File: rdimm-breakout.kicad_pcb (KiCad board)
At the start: 10 copper layers, 152.9 x 45 mm, 33 parts, among them IC1 MIC5317-2.5YM5-TR, IC2 MIC5225-3.3YM5-TR, J1 WE_629105150521, J4 0022232041, U1 FT2232HL-REEL, U14 2199155-1, U8 PCA9517ADMR2G, Y1 KX-7_12,MHz

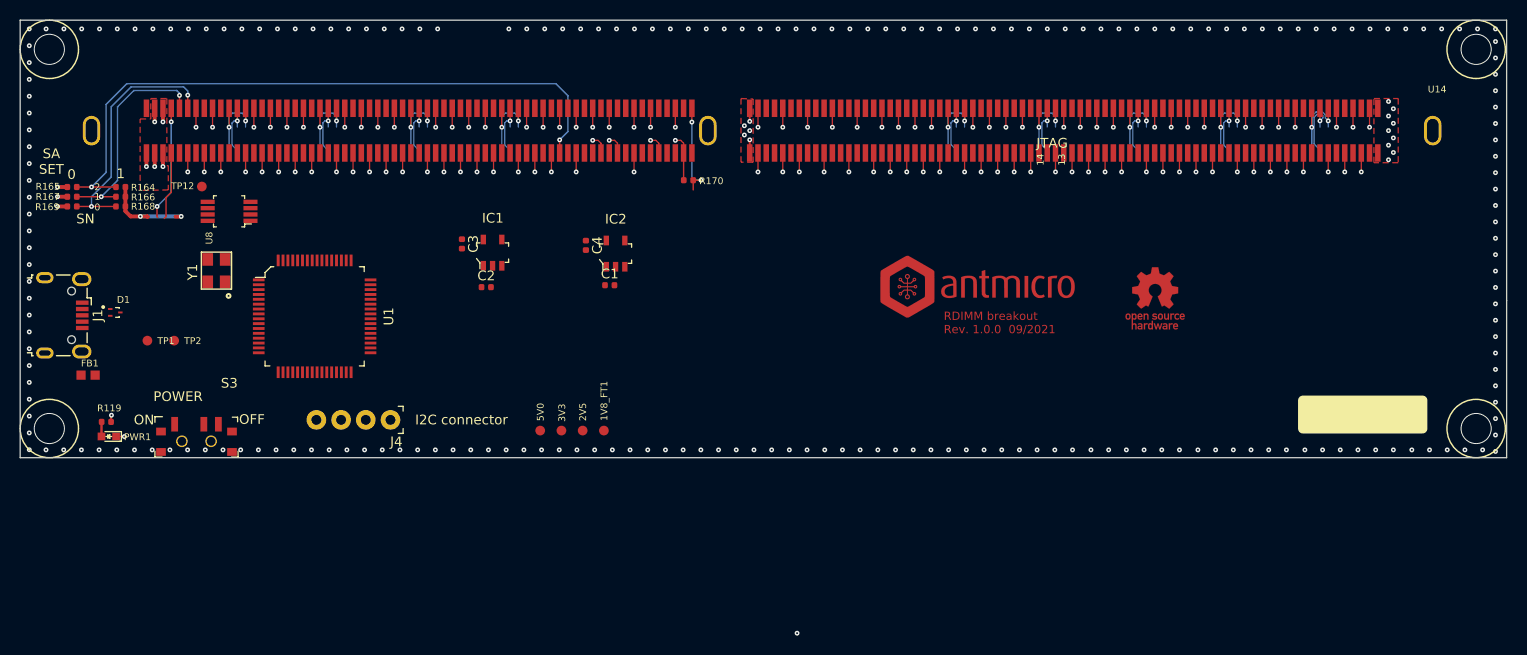
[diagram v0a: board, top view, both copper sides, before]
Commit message: Add layout
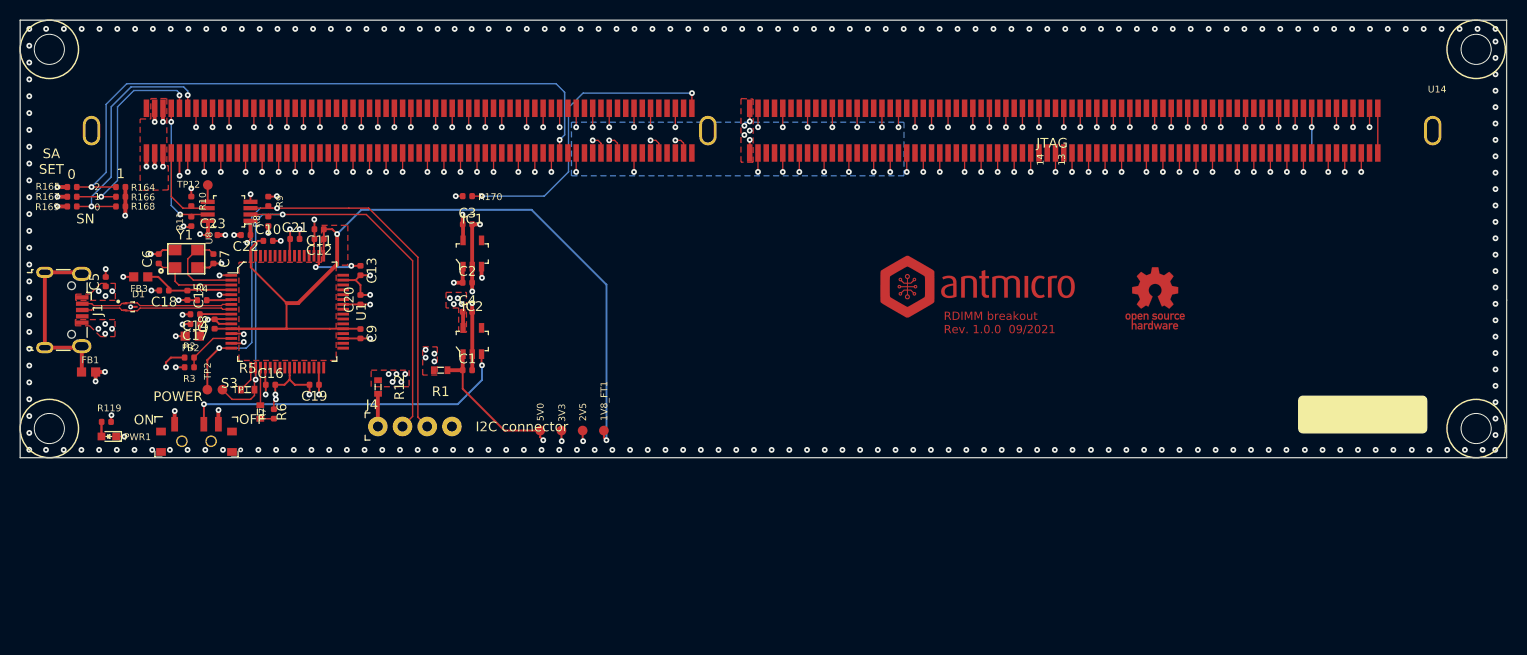
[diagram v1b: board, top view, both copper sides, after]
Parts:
- added C10: C_100n_0402, rdimm-breakout-footprints:0402-cap, F.Cu at (132.5, 68.7)
- added C11: C_100n_0402, rdimm-breakout-footprints:0402-cap, F.Cu at (137.8, 67.5)
- added C12: C_4u7_0402, rdimm-breakout-footprints:0402-cap, F.Cu at (137.8, 68.5)
- added C13: C_100n_0402, rdimm-breakout-footprints:0402-cap, F.Cu at (142.0, 71.8)
- added C14: C_100n_0402, rdimm-breakout-footprints:0402-cap, F.Cu at (125.0, 76.2)
- added C15: C_100n_0402, rdimm-breakout-footprints:0402-cap, F.Cu at (124.2, 74.3)
- added C16: C_100n_0402, rdimm-breakout-footprints:0402-cap, F.Cu at (132.8, 83.5)
- added C17: C_4u7_0402, rdimm-breakout-footprints:0402-cap, F.Cu at (125.0, 77.2)
- added C18: C_4u7_0402, rdimm-breakout-footprints:0402-cap, F.Cu at (121.8, 73.8)
- added C19: C_100n_0402, rdimm-breakout-footprints:0402-cap, F.Cu at (137.2, 83.5)
- added C20: C_100n_0402, rdimm-breakout-footprints:0402-cap, F.Cu at (142.0, 74.8)
- added C21: C_100n_0402, rdimm-breakout-footprints:0402-cap, F.Cu at (135.2, 68.5)
- added C22: C_100n_0402, rdimm-breakout-footprints:0402-cap, F.Cu at (130.2, 68.1)
- added C23: C_100n_0402, rdimm-breakout-footprints:0402-cap, F.Cu at (126.8, 68.1)
- added C5: C_100n_0402, rdimm-breakout-footprints:0402-cap, F.Cu at (115.8, 72.9)
- added C6: C_27p_0402, rdimm-breakout-footprints:0402-cap, F.Cu at (121.3, 70.5)
- added C7: C_27p_0402, rdimm-breakout-footprints:0402-cap, F.Cu at (126.9, 70.5)
- added C8: C_100n_0402, rdimm-breakout-footprints:0402-cap, F.Cu at (127.0, 77.2)
- added C9: C_100n_0402, rdimm-breakout-footprints:0402-cap, F.Cu at (142.0, 78.2)
- added FB2: BLM18AG601SN1D, rdimm-breakout-footprints:0603, F.Cu at (124.7, 78.5)
- added FB3: BLM18AG601SN1D, rdimm-breakout-footprints:0603, F.Cu at (119.4, 72.4)
- added R1: R_0R_0603, rdimm-breakout-footprints:0603-res, F.Cu at (150.2, 82.0)
- added R10: R_10k_0402, rdimm-breakout-footprints:0402-res, F.Cu at (124.6, 64.6)
- added R11: R_10k_0402, rdimm-breakout-footprints:0402-res, F.Cu at (124.6, 66.7)
- added R12: R_0R_0603, rdimm-breakout-footprints:0603-res, F.Cu at (143.8, 83.7)
- added R2: R_4k7_0402, rdimm-breakout-footprints:0402-res, F.Cu at (124.4, 80.7)
- added R3: R_10k_0402, rdimm-breakout-footprints:0402-res, F.Cu at (124.4, 81.7)
- added R4: R_12k_0402, rdimm-breakout-footprints:0402-res, F.Cu at (125.7, 74.8)
- added R5: R_0R_0603, rdimm-breakout-footprints:0603-res, F.Cu at (130.4, 84.0)
- added R6: R_0R_0603, rdimm-breakout-footprints:0603-res, F.Cu at (131.7, 86.3)
- added R7: R_220R_0402, rdimm-breakout-footprints:0402-res, F.Cu at (133.1, 86.5)
- added R8: R_10k_0402, rdimm-breakout-footprints:0402-res, F.Cu at (132.5, 66.7)
- added R9: R_10k_0402, rdimm-breakout-footprints:0402-res, F.Cu at (132.5, 64.6)
- moved R170 22.8 mm to (153.0, 64.1)
- moved IC2 17.3 mm to (153.5, 79.0)
- moved C1 17.0 mm to (153.0, 82.0)
- moved C4 14.0 mm to (153.0, 76.0), turned to 0 degrees
- moved TP1 9.21 mm to (127.8, 83.9)
- moved TP2 6.10 mm to (126.2, 84.0), turned to 270 degrees
- moved Y1 3.37 mm to (124.0, 70.5), turned to 0 degrees
- moved U1 2.86 mm to (134.5, 76.0)
- moved IC1 2.09 mm to (153.5, 70.0)
- moved C3 2.09 mm to (153.0, 67.0), turned to 0 degrees
- moved C2 1.99 mm to (153.0, 73.0)
- moved D1 1.65 mm to (118.3, 75.5)
- moved J4 1.47 mm to (143.8, 87.8), turned to 0 degrees
- moved TP12 0.63 mm to (126.3, 62.9)
- moved J1 0.55 mm to (111.5, 75.8)
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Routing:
- net (no net): track 125.3 -> 0.00 mm, vias 72 -> 4
- net 1V8_FT: track 0.00 -> 95.5 mm, vias 0 -> 2
- net GND: track 200.7 -> 271.2 mm, vias 262 -> 357
- net SDA: track 0.00 -> 62.9 mm, vias 0 -> 2
- net SCL: track 0.00 -> 62.5 mm, vias 0 -> 2
- net /FTDI/3V3_EN: track 0.00 -> 34.4 mm, vias 0 -> 2
- net VCC3V3: track 0.86 -> 34.5 mm, vias 4 -> 26
- net ~EVENT: track 10.1 -> 32.4 mm
- net Net-(FB1-Pad1): track 0.00 -> 18.1 mm
- net VCC5V0: track 0.00 -> 16.0 mm, vias 0 -> 1
- net /FTDI/USB_D_N: track 0.00 -> 15.7 mm
- net /FTDI/USB_D_P: track 0.00 -> 15.7 mm
- net OSCI: track 0.00 -> 9.51 mm
- net Net-(C15-Pad1): track 0.00 -> 9.40 mm
- net OSCO: track 0.00 -> 9.21 mm
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- added copper zone on F.Cu, net 1V8_FT
- added copper zone on F.Cu, net GND
- added copper zone on F.Cu, net VBUS
- added copper zone on VCC, net VBUS
- added copper zone on VCC, net VCC2V5
- added copper zone on F.Cu, net VCC3V3
- added copper zone on VCC, net VCC3V3
- added copper zone on B.Cu, net VDDQ
- removed copper zone on VCC2, net 1V0_SYS
- removed copper zone on VCC1, net 1V2_SYS
- removed copper zone on VCC1, net 1V8_FT
- removed copper zone on VCC2, net 1V8_SYS
- removed copper zone on VCC1, net 3V3_SYS
- removed copper zone on GND2, net GND
- removed copper zone on F.Cu, net NC
- removed copper zone on VCC2, net NC
- removed copper zone on VCC2, net VCC5V0
- removed copper zone on VCC1, net VDDQ
- removed copper zone on VCC2, net VIN
- removed copper zone on VCC2, net VPP
- removed copper zone on VCC2, net VTT
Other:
- copper layers 10 -> 4
- rule via_min_size: 0.45 -> 0.4
